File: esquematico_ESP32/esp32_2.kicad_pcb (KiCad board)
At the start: 2 copper layers, 79.6 x 93.5 mm, 39 parts, among them J2 Conn_RFID1, J3 Conn_RFID2, J4 USB_A, J5 Conn_screen, J6 Conn_01x04_Female, J7 Jack-DC, Q1 BSS138, Q2 BSS138, SW1 SW_Push, SW2 Enable, U1 ESP32-WROOM-32, U2 LM1117-3.3, U3 LM2596S-5

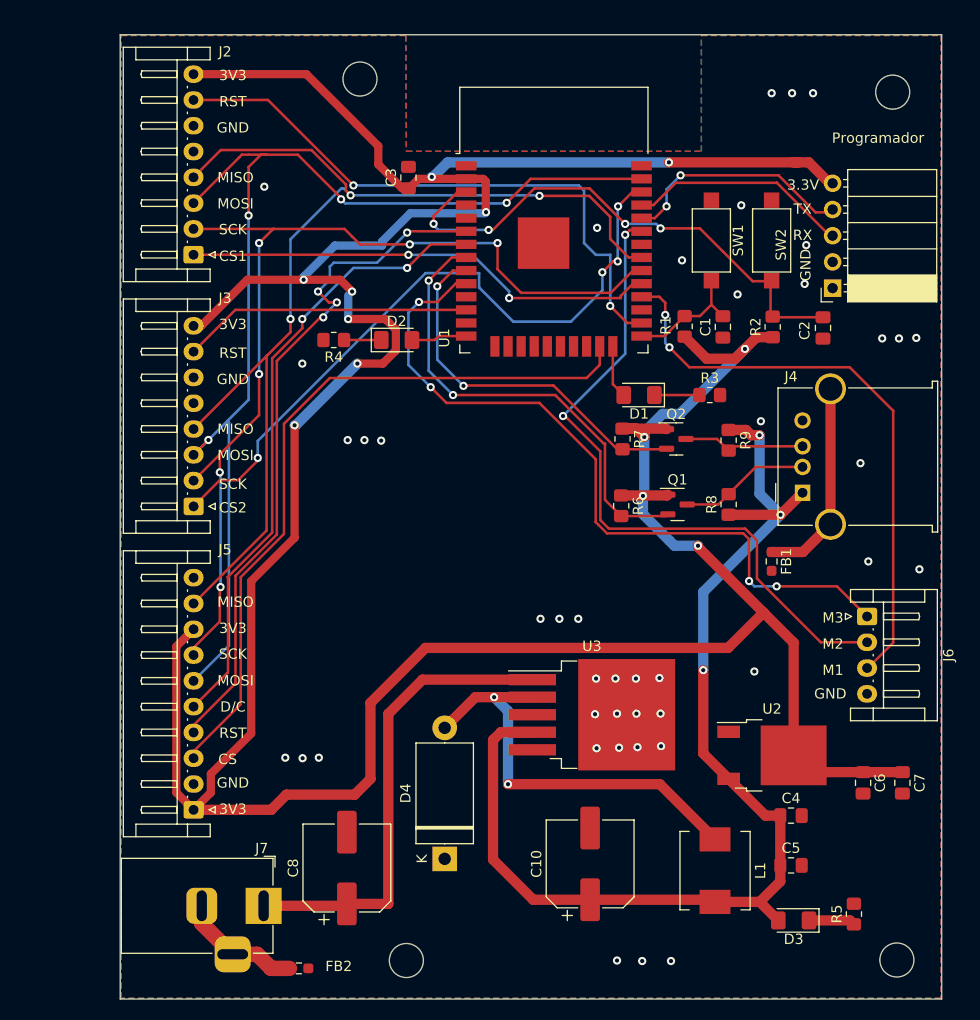
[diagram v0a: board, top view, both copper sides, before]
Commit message: Alternativa_Acomodada
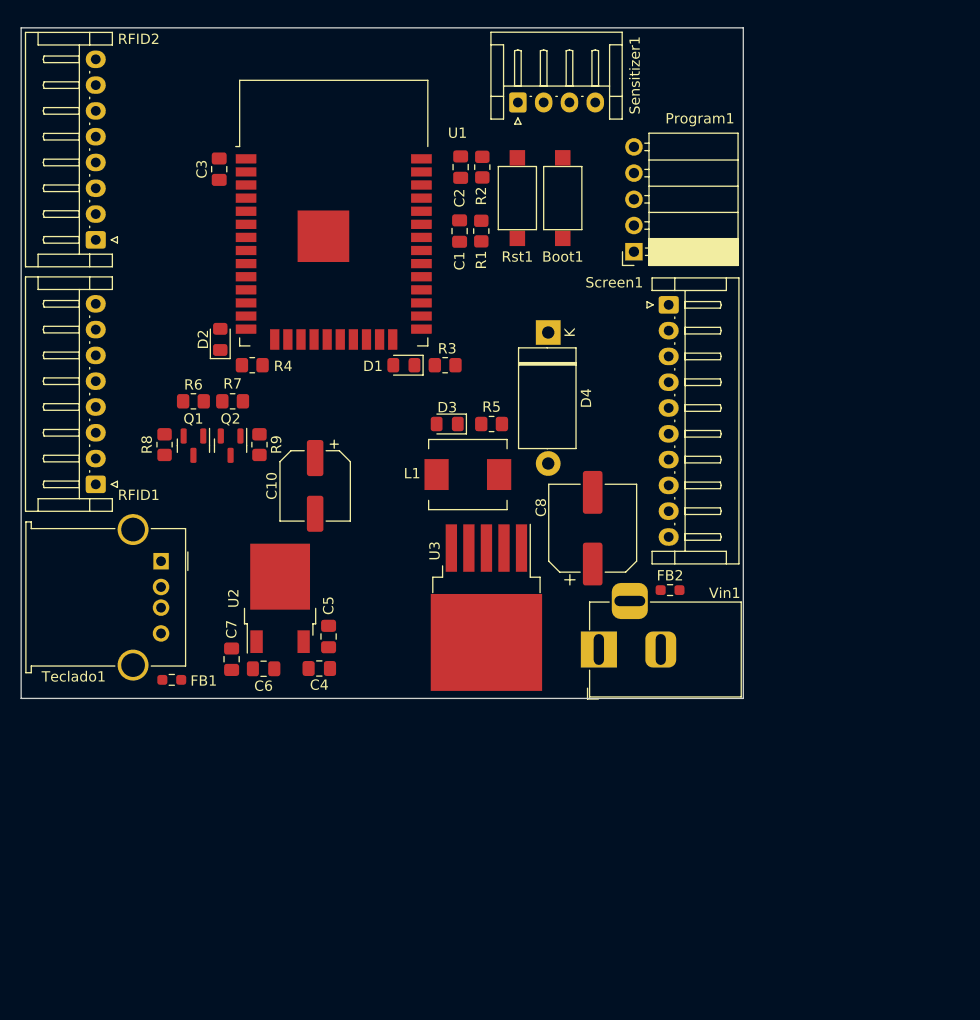
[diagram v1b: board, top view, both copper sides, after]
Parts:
- removed J2: Conn_RFID1, Connector_JST:JST_EH_S8B-EH_1x08_P2.50mm_Horizontal
- removed J3: Conn_RFID2, Connector_JST:JST_EH_S8B-EH_1x08_P2.50mm_Horizontal
- removed J4: USB_A, Connector_USB:USB_A_Molex_67643_Horizontal
- removed J5: Conn_screen, Connector_JST:JST_EH_S10B-EH_1x10_P2.50mm_Horizontal
- removed J6: Conn_01x04_Female, Connector_JST:JST_EH_S4B-EH_1x04_P2.50mm_Horizontal
- removed J7: Jack-DC, Connector_BarrelJack:BarrelJack_Horizontal
- removed Programador: programador, Connector_PinSocket_2.54mm:PinSocket_1x05_P2.54mm_Horizontal
- removed SW1: SW_Push, Button_Switch_SMD:SW_SPST_CK_RS282G05A3
- removed SW2: Enable, Button_Switch_SMD:SW_SPST_CK_RS282G05A3
- added Boot1: SW_Push, Button_Switch_SMD:SW_SPST_CK_RS282G05A3, F.Cu at (173.2, 43.9)
- added Program1: Conn_01x05_Female, Connector_PinSocket_2.54mm:PinSocket_1x05_P2.54mm_Horizontal, F.Cu at (180.1, 49.1)
- added RFID1: J2, Connector_JST:JST_EH_S8B-EH_1x08_P2.50mm_Horizontal, F.Cu at (127.9, 71.7)
- added RFID2: J3, Connector_JST:JST_EH_S8B-EH_1x08_P2.50mm_Horizontal, F.Cu at (127.9, 48.0)
- added Rst1: Enable, Button_Switch_SMD:SW_SPST_CK_RS282G05A3, F.Cu at (168.8, 43.9)
- added Screen1: J5, Connector_JST:JST_EH_S10B-EH_1x10_P2.50mm_Horizontal, F.Cu at (183.5, 54.2)
- added Sensitizer1: Conn_01x04_Female, Connector_JST:JST_EH_S4B-EH_1x04_P2.50mm_Horizontal, F.Cu at (168.8, 34.6)
- added Teclado1: USB_A, Connector_USB:USB_A_Molex_67643_Horizontal, F.Cu at (134.3, 79.1)
- added Vin1: Jack-DC, Connector_BarrelJack:BarrelJack_Horizontal, F.Cu at (176.7, 87.7)
- C10: footprint Capacitor_SMD:CP_Elec_8x6.9 -> Capacitor_SMD:CP_Elec_6.3x7.7
- D1, D2, D3: footprint LED_SMD:LED_1206_3216Metric_Pad1.42x1.75mm_HandSolder -> LED_SMD:LED_0805_2012Metric_Pad1.15x1.40mm_HandSolder
- moved C7 66.1 mm to (141.1, 88.6)
- moved FB1 59.3 mm to (135.3, 90.6), turned to 0 degrees
- moved C6 59.2 mm to (144.2, 89.5), turned to 180 degrees
- moved R5 59.1 mm to (166.3, 65.8), turned to 0 degrees
- moved D3 58.7 mm to (162.0, 65.8)
- moved R8 55.0 mm to (134.6, 67.8), turned to -90 degrees
- moved D4 52.0 mm to (171.7, 57.0), turned to -90 degrees
- moved FB2 51.4 mm to (183.6, 81.9)
- moved U2 50.0 mm to (145.8, 82.7), turned to 90 degrees
- moved C5 50.0 mm to (150.5, 86.4), turned to 90 degrees
- moved C4 47.9 mm to (149.6, 89.5), turned to 180 degrees
- moved Q1 47.3 mm to (137.4, 67.9), turned to -90 degrees
- moved R9 45.5 mm to (143.8, 67.8)
- moved C10 45.3 mm to (149.2, 71.8), turned to -90 degrees
- moved L1 45.3 mm to (164.0, 70.7), turned to 180 degrees
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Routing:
- net +3V3: track 351.4 -> 0.00 mm, vias 12 -> 0
- net +5V: track 111.0 -> 0.00 mm, vias 3 -> 0
- net /MOSI: track 109.4 -> 0.00 mm, vias 4 -> 0
- net /MISO: track 107.8 -> 0.00 mm, vias 3 -> 0
- net /SCK: track 97.0 -> 0.00 mm, vias 6 -> 0
- net /MAGNE_3: track 72.3 -> 0.00 mm, vias 4 -> 0
- net /CS_Display: track 70.8 -> 0.00 mm
- net /RST_D: track 67.4 -> 0.00 mm, vias 4 -> 0
- net /MAGNE_2: track 66.5 -> 0.00 mm, vias 2 -> 0
- net /CS_LECTOR_2: track 66.0 -> 0.00 mm, vias 4 -> 0
- net /D/C: track 60.9 -> 0.00 mm, vias 2 -> 0
- net /RST_1: track 58.3 -> 0.00 mm, vias 2 -> 0
- net /MAGNE_1: track 57.3 -> 0.00 mm, vias 2 -> 0
- net /EN: track 51.7 -> 0.00 mm, vias 4 -> 0
- net /CS_LECTOR_1: track 46.2 -> 0.00 mm, vias 2 -> 0
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- removed copper zone on B.Cu, net GND
- removed copper zone on F.Cu, net GND
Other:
- board size 79.6 x 93.5 mm -> 70 x 65 mm
- board text removed: "3.3V"
- board text removed: "3V3"
- board text removed: "CS"
- board text removed: "CS1"
- board text removed: "CS2"
- board text removed: "D/C"
- board text removed: "GND"
- board text removed: "M1"
- board text removed: "M2"
- board text removed: "M3"
- board text removed: "MISO"
- board text removed: "MOSI"
- board text removed: "RST"
- board text removed: "RX"
- board text removed: "SCK"
- board text removed: "TX"
